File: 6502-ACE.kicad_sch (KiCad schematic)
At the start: 156 parts, among them J10 RESET SW, J11 6502 CART, J12 6502 BUS, J13 PADDLES, J14 AUDIO L, J15 AUDIO R, J16 Compact Flash, J17 DB9 MALE (DTE), J18 CTS EN, J19 DCD EN, J2 PHI2 Select, J20 ACT LED, J21 IDE, J3 PS/2, J4 JOYSTICK A, J5 JOYSTICK B, J6 PORT B, J7 PORT B, J8 PORT A, J9 PORT A, SW1 `, SW10 1, SW11 9, SW12 W, SW13 P, SW14 D, SW15 ', SW16 B, SW17 MENU, SW18 2, SW19 0, SW2 8, SW20 E, SW21 [, SW22 F, SW23 ENTER, SW24 N, SW25 ALT, SW26 R ALT, SW27 3, SW28 -, SW29 R, SW3 Q, SW30 ], SW31 G, SW32 DELETE, SW33 M, SW34 SPACE, SW35 4, SW36 =, SW37 T, SW38 \, SW39 H, SW4 O, SW40 SHIFT, SW41 R SHIFT, SW42 ,, SW43 FN, SW44 5, SW45 BACKSPACE, SW46 Y, SW47 INSERT, SW48 J, SW49 Z, SW5 S, SW50 ., SW51 LEFT ARROW, SW52 6, SW53 ESCAPE, SW54 U, SW55 CAPS LOCK, SW56 K, SW57 X, SW58 /, SW59 DOWN ARROW, SW6 ;, SW60 7, SW61 TAB, SW62 I, SW63 A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

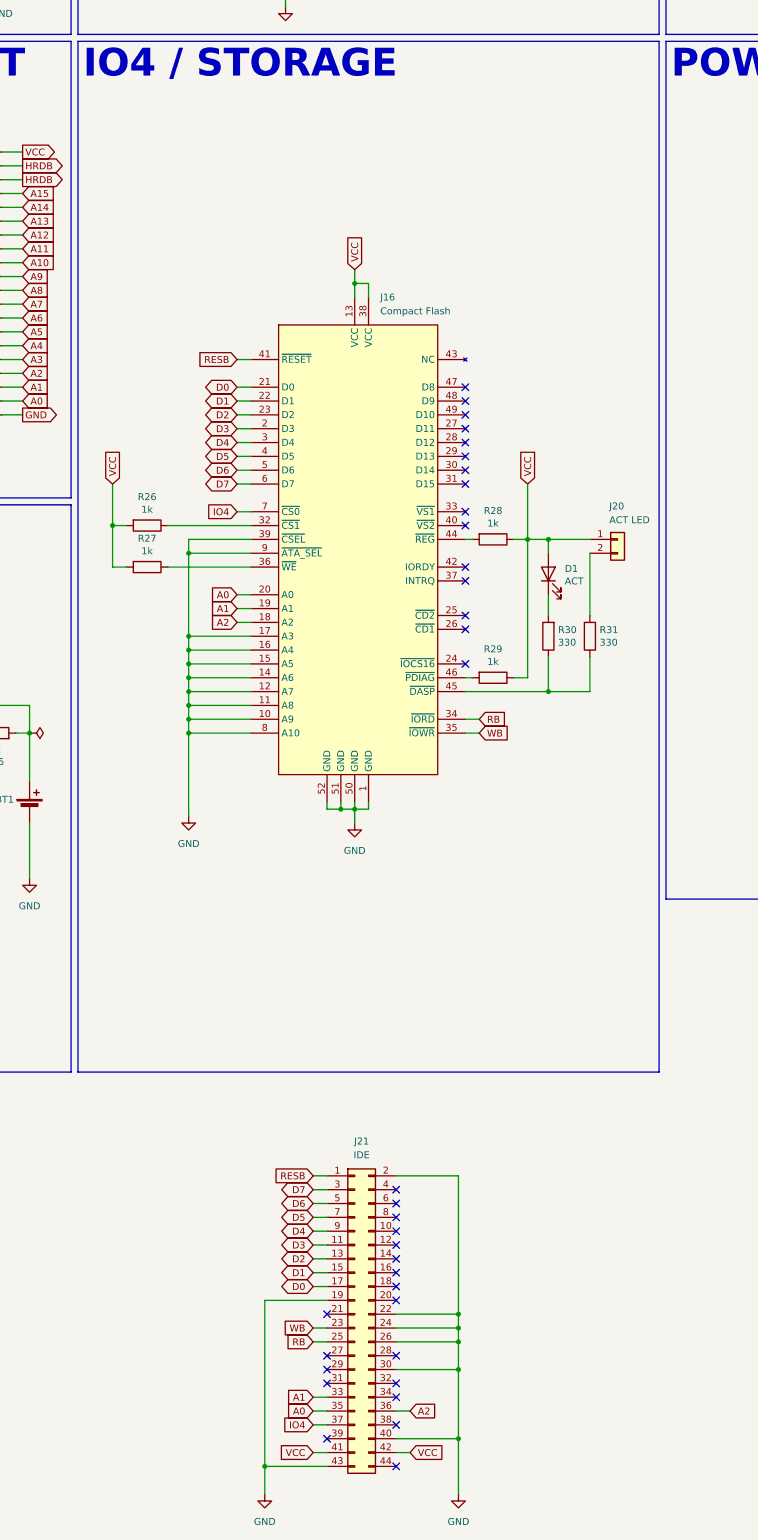
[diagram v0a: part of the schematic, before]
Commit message: Update PDF
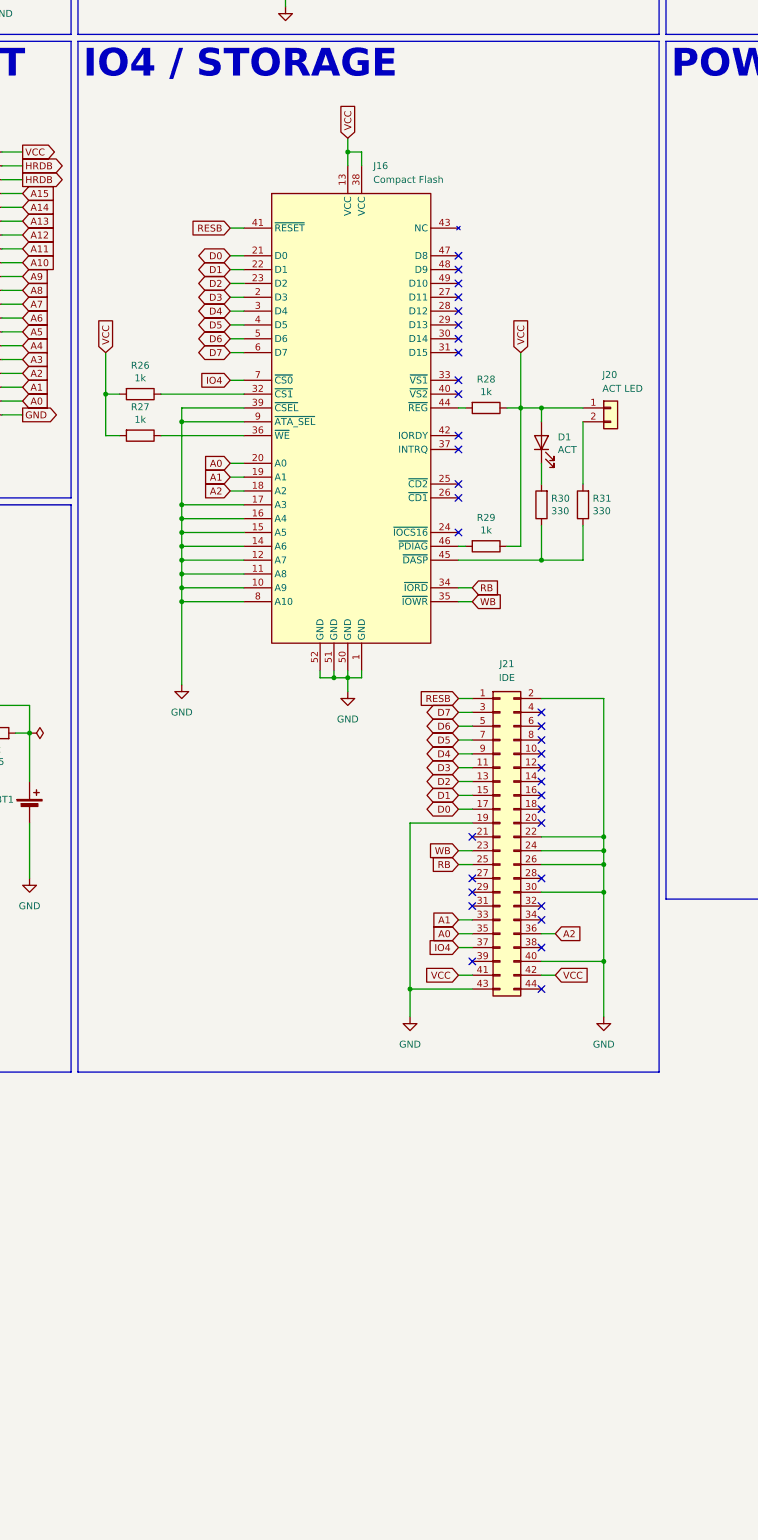
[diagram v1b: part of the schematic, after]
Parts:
- added unit 1 of U1
- added unit 5 of U14
- added unit 2 of U15
- added unit 5 of U16
- added unit 1 of U5
- added unit 1 of U6
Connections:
- net A14: now also U1.1, U1.2, U6.2; no longer U1.1, U1.2, U6.2
- net GND: now also U14.7 (GND), U15.7 (GND), U16.7 (GND); no longer U14.7 (GND), U15.7 (GND), U16.7 (GND)
- net HRDB: now also U6.1; no longer U6.1
- net REB: now also U5.3; no longer U5.3
- net VCC: now also U14.14 (VCC), U15.14 (VCC), U16.14 (VCC); no longer U14.14 (VCC), U15.14 (VCC), U16.14 (VCC)
- net at U1.4: now also U1.3; no longer U1.3
- net at U6.4, U6.5: now also U6.3; no longer U6.3
- new net: U5.1, U5.2, U6.11
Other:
- moved on the sheet: D1, J16, J20, J21, R26, R27, R28, R29, R30, R31
